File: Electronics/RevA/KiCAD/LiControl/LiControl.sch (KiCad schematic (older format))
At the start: 81 parts, among them J1 Conn_01x07, J2 Conn_01x06, J4 Conn_01x07, J5 RJ45, Q1 Q_NMOS_GSD, Q10 Q_NMOS_GSD, Q11 Q_PMOS_GSD, Q12 Q_NMOS_GSD, Q2 Q_NMOS_GSD, Q3 Q_NMOS_GSD, Q4 Q_NMOS_GSD, Q5 Q_NMOS_GSD, Q6 Q_NMOS_GSD, Q7 Q_PMOS_GSD, Q8 Q_PMOS_GSD, Q9 Q_PMOS_GSD

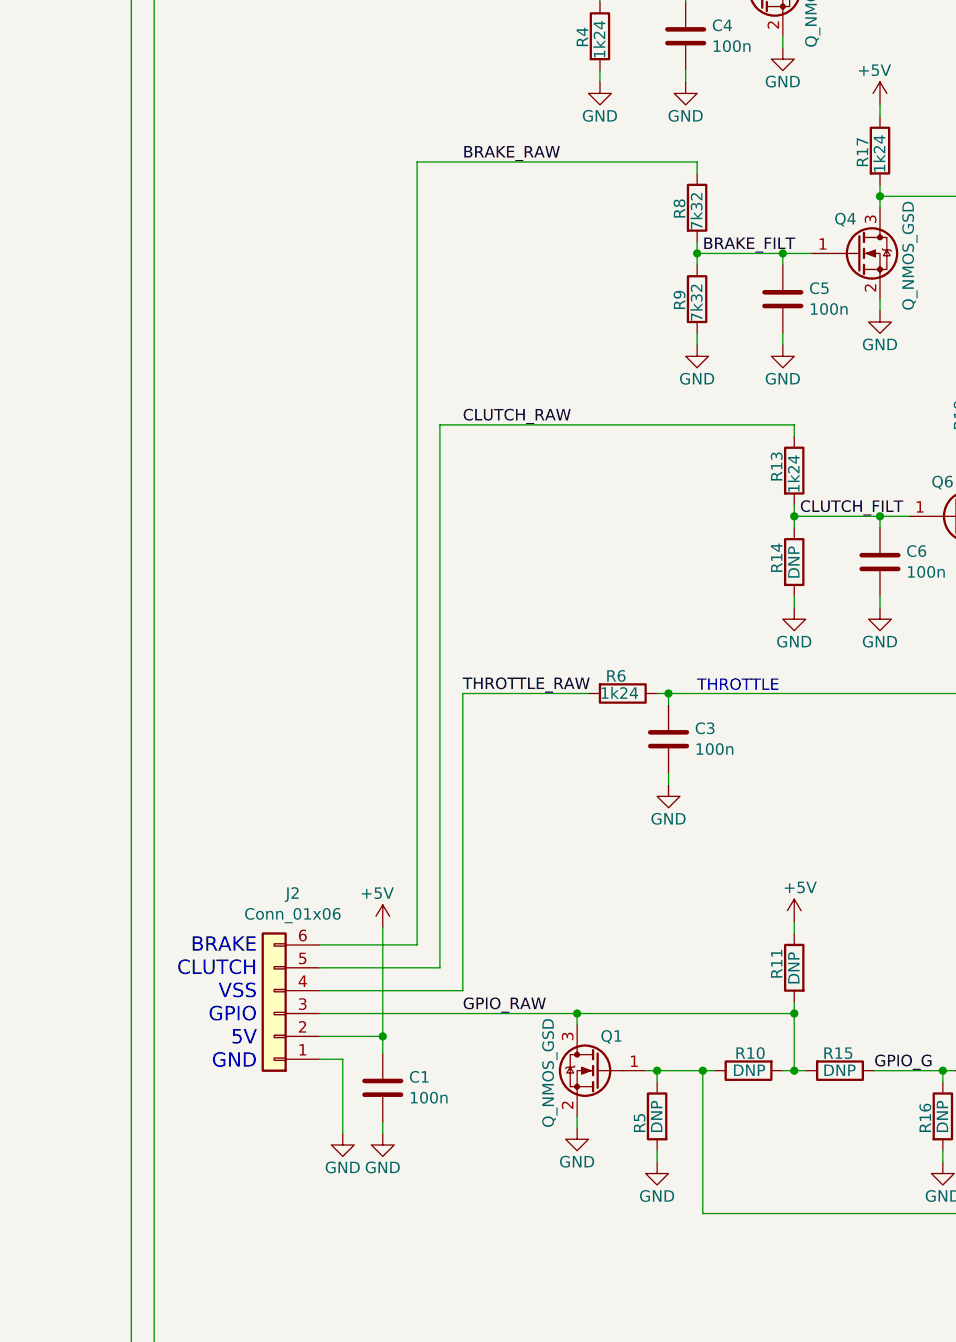
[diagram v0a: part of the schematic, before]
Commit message: Final RevA PCB
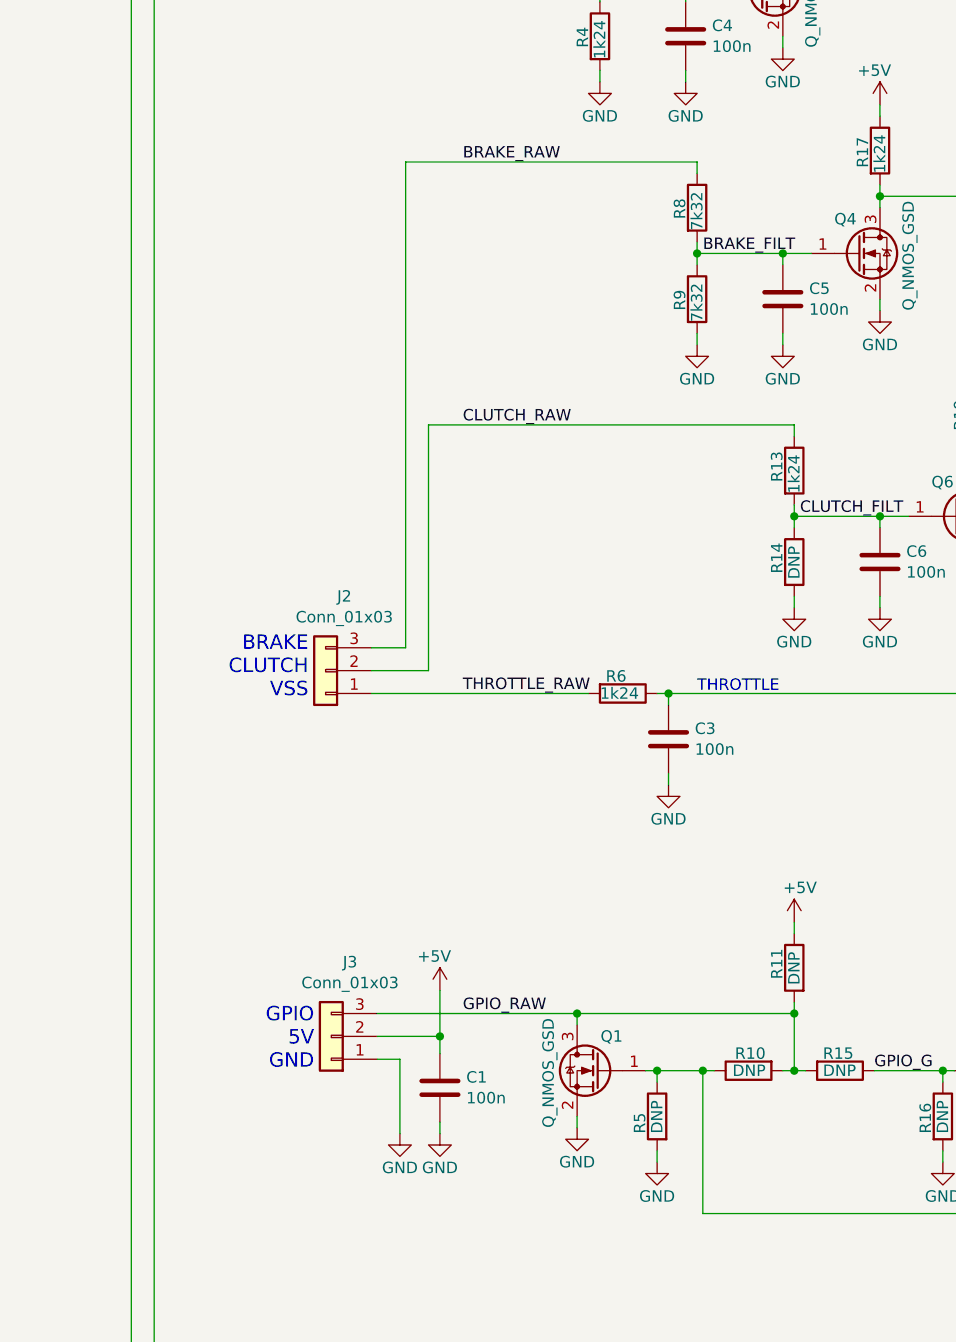
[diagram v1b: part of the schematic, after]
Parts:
- removed J2: Conn_01x06, Connector_Phoenix_MC:PhoenixContact_MC_1,5_6-G-3.5_1x06_P3.50mm_Horizontal, symbol Connector_Generic:Conn_01x06
- added J2, J3: Conn_01x03, Connector_Phoenix_MC:PhoenixContact_MCV_1,5_3-G-3.5_1x03_P3.50mm_Vertical, symbol Connector_Generic:Conn_01x03
- J1, J4: footprint Connector_Phoenix_MC:PhoenixContact_MC_1,5_7-G-3.5_1x07_P3.50mm_Horizontal -> Connector_Phoenix_MC:PhoenixContact_MCV_1,5_7-G-3.5_1x07_P3.50mm_Vertical
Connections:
- net +5V: now also J3.2 (Pin_2)
- net BRAKE_RAW: now also J2.3 (Pin_3)
- net CLUTCH_RAW: now also J2.2 (Pin_2)
- net GND: now also J3.1 (Pin_1)
- net GPIO_RAW: now also J3.3 (Pin_3)
- net THROTTLE_RAW: now also J2.1 (Pin_1)
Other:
- note added: "BRAKE\nCLUTCH\nVSS"
- note added: "GPIO\n5V\nGND"
- note removed: "BRAKE\nCLUTCH\nVSS\nGPIO\n5V\nGND"
- moved on the sheet: C1
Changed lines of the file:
@@
 F 0 "J1" H 2775 1475 50  0000 C CNN
 F 1 "Conn_01x07" H 2775 2275 50  0000 C CNN
-F 2 "Connector_Phoenix_MC:PhoenixContact_MC_1,5_7-G-3.5_1x07_P3.50mm_Horizontal" H 2775 1875 50  0001 C CNN
+F 2 "Connector_Phoenix_MC:PhoenixContact_MCV_1,5_7-G-3.5_1x07_P3.50mm_Vertical" H 2775 1875 50  0001 C CNN
 F 3 "~" H 2775 1875 50  0001 C CNN
 	1    2775 1875
@@
 F 0 "J4" H 10925 2275 50  0000 C CNN
 F 1 "Conn_01x07" H 10925 1475 50  0000 C CNN
-F 2 "Connector_Phoenix_MC:PhoenixContact_MC_1,5_7-G-3.5_1x07_P3.50mm_Horizontal" H 10925 1875 50  0001 C CNN
+F 2 "Connector_Phoenix_MC:PhoenixContact_MCV_1,5_7-G-3.5_1x07_P3.50mm_Vertical" H 10925 1875 50  0001 C CNN
 F 3 "~" H 10925 1875 50  0001 C CNN
 	1    10925 1875
@@
 	7475 6075 7475 8675
 $Comp
-L Connector_Generic:Conn_01x06 J2
-U 1 1 65587D5B
-P 3875 8675
-F 0 "J2" H 3793 8150 50  0000 C CNN
-F 1 "Conn_01x06" H 3793 8241 50  0000 C CNN
-F 2 "Connector_Phoenix_MC:PhoenixContact_MC_1,5_6-G-3.5_1x06_P3.50mm_Horizontal" H 3875 8675 50  0001 C CNN
-F 3 "~" H 3875 8675 50  0001 C CNN
-	1    3875 8675
-	-1   0    0    1
-$EndComp
-$Comp
 L Device:C C1
 U 1 1 655D5C67
-P 4350 9000
-F 0 "C1" H 4235 8954 50  0000 R CNN
-F 1 "100n" H 4235 9045 50  0000 R CNN
-F 2 "Capacitor_SMD:C_0805_2012Metric" H 4388 8850 50  0001 C CNN
-F 3 "~" H 4350 9000 50  0001 C CNN
-	1    4350 9000
+P 4600 9000
+F 0 "C1" H 4485 8954 50  0000 R CNN
+F 1 "100n" H 4485 9045 50  0000 R CNN
+F 2 "Capacitor_SMD:C_0805_2012Metric" H 4638 8850 50  0001 C CNN
+F 3 "~" H 4600 9000 50  0001 C CNN
+	1    4600 9000
 	-1   0    0    1
 $EndComp
 Wire Wire Line
-	4350 9150 4350 9200
+	4600 9150 4600 9200
 $Comp
 L power:GND #PWR04
 U 1 1 655D5C6E
-P 4350 9200
-F 0 "#PWR04" H 4350 8950 50  0001 C CNN
-F 1 "GND" H 4350 9050 50  0000 C CNN
-F 2 "" H 4350 9200 50  0001 C CNN
-F 3 "" H 4350 9200 50  0001 C CNN
-	1    4350 9200
+P 4600 9200
+F 0 "#PWR04" H 4600 8950 50  0001 C CNN
+F 1 "GND" H 4600 9050 50  0000 C CNN
+F 2 "" H 4600 9200 50  0001 C CNN
+F 3 "" H 4600 9200 50  0001 C CNN
+	1    4600 9200
 	1    0    0    -1
 $EndComp
@@
 L power:GND #PWR02
 U 1 1 65606C81
-P 4175 9200
-F 0 "#PWR02" H 4175 8950 50  0001 C CNN
-F 1 "GND" H 4175 9050 50  0000 C CNN
-F 2 "" H 4175 9200 50  0001 C CNN
-F 3 "" H 4175 9200 50  0001 C CNN
-	1    4175 9200
-	1    0    0    -1
-$EndComp
-Wire Wire Line
-	4175 9200 4175 8875
-Wire Wire Line
-	4175 8875 4075 8875
-Wire Wire Line
-	4075 8775 4350 8775
-Wire Wire Line
-	4075 8375 4500 8375
-Wire Wire Line
-	4500 8375 4500 4950
-Wire Wire Line
-	4500 4950 5725 4950
-Wire Wire Line
-	4600 6100 4600 8475
-Wire Wire Line
-	4600 8475 4075 8475
-Wire Wire Line
-	4600 6100 6150 6100
-Wire Wire Line
-	4075 8575 4700 8575
-Wire Wire Line
-	4700 8575 4700 7275
-Wire Wire Line
-	4700 7275 5250 7275
+P 4425 9200
+F 0 "#PWR02" H 4425 8950 50  0001 C CNN
+F 1 "GND" H 4425 9050 50  0000 C CNN
+F 2 "" H 4425 9200 50  0001 C CNN
+F 3 "" H 4425 9200 50  0001 C CNN
+	1    4425 9200
+	1    0    0    -1
+$EndComp
+Wire Wire Line
+	4425 9200 4425 8875
+Wire Wire Line
+	4425 8875 4325 8875
+Wire Wire Line
+	4325 8775 4600 8775
 $Comp
 L Device:R R15
@@
 L power:+5V #PWR03
 U 1 1 65B6E1CD
-P 4350 8300
-F 0 "#PWR03" H 4350 8150 50  0001 C CNN
-F 1 "+5V" H 4325 8450 50  0000 C CNN
-F 2 "" H 4350 8300 50  0001 C CNN
-F 3 "" H 4350 8300 50  0001 C CNN
-	1    4350 8300
+P 4600 8575
+F 0 "#PWR03" H 4600 8425 50  0001 C CNN
+F 1 "+5V" H 4575 8725 50  0000 C CNN
+F 2 "" H 4600 8575 50  0001 C CNN
+F 3 "" H 4600 8575 50  0001 C CNN
+	1    4600 8575
 	1    0    0    -1
 $EndComp
@@
 Connection ~ 6800 8925
 Wire Wire Line
-	4350 8775 4350 8850
-Wire Wire Line
-	4350 8775 4350 8300
-Connection ~ 4350 8775
+	4600 8775 4600 8850
+Wire Wire Line
+	4600 8775 4600 8575
+Connection ~ 4600 8775
 Wire Wire Line
 	6100 3900 6100 3950
@@
 Wire Wire Line
 	6100 3950 6100 4000
-Text Notes 3800 8925 2    63   ~ 0
-BRAKE\nCLUTCH\nVSS\nGPIO\n5V\nGND
+Text Notes 4050 8925 2    63   ~ 0
+GPIO\n5V\nGND
 Wire Wire Line
 	7675 8300 7675 10475
@@
 	5200 8675 6150 8675
 Wire Wire Line
-	4075 8675 5200 8675
+	4325 8675 5200 8675
 Wire Wire Line
 	5750 8925 5550 8925
@@
 	9800 3425 9800 5225
 NoConn ~ 9700 3525
+$Comp
+L Connector_Generic:Conn_01x03 J2
+U 1 1 63F787FB
+P 4100 7175
+F 0 "J2" H 4018 6850 50  0000 C CNN
+F 1 "Conn_01x03" H 4018 6941 50  0000 C CNN
+F 2 "Connector_Phoenix_MC:PhoenixContact_MCV_1,5_3-G-3.5_1x03_P3.50mm_Vertical" H 4100 7175 50  0001 C CNN
+F 3 "~" H 4100 7175 50  0001 C CNN
+	1    4100 7175
+	-1   0    0    1
+$EndComp
+Wire Wire Line
+	4300 7275 5250 7275
+Wire Wire Line
+	4300 7175 4550 7175
+Wire Wire Line
+	4550 7175 4550 6100
+Wire Wire Line
+	4550 6100 6150 6100
+Wire Wire Line
+	4300 7075 4450 7075
+Wire Wire Line
+	4450 7075 4450 4950
+Wire Wire Line
+	4450 4950 5725 4950
+Text Notes 4025 7300 2    63   ~ 0
+BRAKE\nCLUTCH\nVSS
+$Comp
+L Connector_Generic:Conn_01x03 J3
+U 1 1 6403BC2E
+P 4125 8775
+F 0 "J3" H 4043 8450 50  0000 C CNN
+F 1 "Conn_01x03" H 4043 8541 50  0000 C CNN
+F 2 "Connector_Phoenix_MC:PhoenixContact_MCV_1,5_3-G-3.5_1x03_P3.50mm_Vertical" H 4125 8775 50  0001 C CNN
+F 3 "~" H 4125 8775 50  0001 C CNN
+	1    4125 8775
+	-1   0    0    1
+$EndComp
 $EndSCHEMATC
